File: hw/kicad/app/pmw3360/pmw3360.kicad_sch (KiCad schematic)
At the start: 13 parts, among them J1 TOP, J2 BUTTOM, U1 PMW3360DM-T2QU, U2 AMS1117-1.8

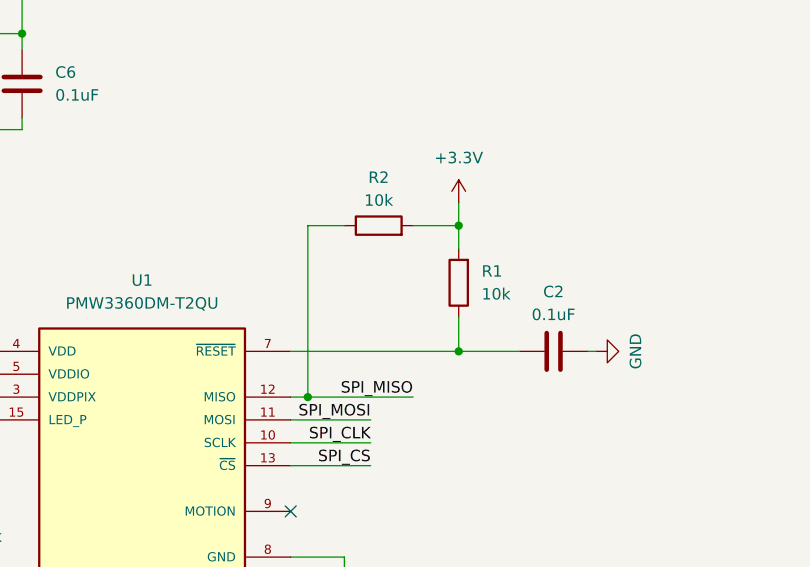
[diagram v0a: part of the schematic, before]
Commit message: Merge from normal
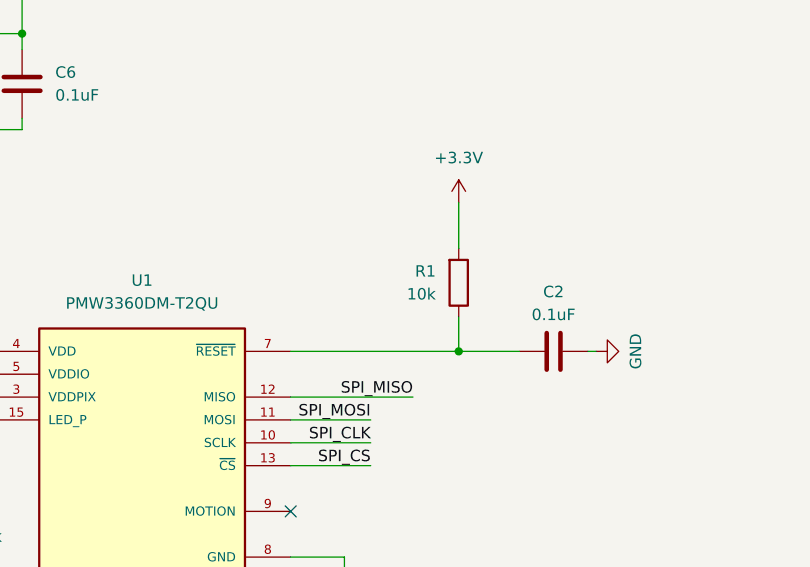
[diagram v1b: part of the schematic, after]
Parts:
- removed R2: 10k, Resistor_SMD:R_0805_2012Metric, symbol Device:R
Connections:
- net GND: now also C2.1; no longer C2.2
- net at R1.1, U1.7 (~{RESET}): now also C2.2; no longer C2.1
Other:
- moved on the sheet: C2, R1
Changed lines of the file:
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@@
 (kicad_sch (version 20230121) (generator eeschema)
   (paper "A4")
-  (junction (at 121.666 83.82) (diameter 0) (color 0 0 0 0)
-  )
   (junction (at 74.676 107.442) (diameter 0) (color 0 0 0 0)
   )
@@
   )
   (junction (at 89.916 43.434) (diameter 0) (color 0 0 0 0)
-  )
-  (junction (at 138.43 64.77) (diameter 0) (color 0 0 0 0)
   )
   (no_connect (at 119.761 96.52))
@@
     (stroke (width 0) (type default))
   )
-  (wire (pts (xy 133.35 83.82) (xy 121.666 83.82))
+  (wire (pts (xy 119.761 83.82) (xy 133.35 83.82))
     (stroke (width 0) (type default))
   )
@@
     (stroke (width 0) (type default))
   )
-  (wire (pts (xy 121.666 83.82) (xy 121.666 64.77))
-    (stroke (width 0) (type default))
-  )
   (wire (pts (xy 77.978 54.102) (xy 89.916 54.102))
     (stroke (width 0) (type default))
@@
     (stroke (width 0) (type default))
   )
-  (wire (pts (xy 133.35 64.77) (xy 138.43 64.77))
-    (stroke (width 0) (type default))
-  )
   (wire (pts (xy 231.14 80.01) (xy 240.03 80.01))
     (stroke (width 0) (type default))
@@
     (stroke (width 0) (type default))
   )
-  (wire (pts (xy 138.43 62.23) (xy 138.43 64.77))
+  (wire (pts (xy 138.43 62.23) (xy 138.43 67.31))
     (stroke (width 0) (type default))
   )
@@
     (stroke (width 0) (type default))
   )
-  (wire (pts (xy 121.666 64.77) (xy 125.73 64.77))
-    (stroke (width 0) (type default))
-  )
   (wire (pts (xy 224.79 85.09) (xy 215.9 85.09))
     (stroke (width 0) (type default))
@@
     (stroke (width 0) (type default))
   )
-  (wire (pts (xy 138.43 64.77) (xy 138.43 67.31))
-    (stroke (width 0) (type default))
-  )
   (wire (pts (xy 119.761 78.74) (xy 138.43 78.74))
     (stroke (width 0) (type default))
@@
     (stroke (width 0) (type default))
   )
-  (wire (pts (xy 121.666 83.82) (xy 119.761 83.82))
-    (stroke (width 0) (type default))
-  )
   (wire (pts (xy 63.5 41.656) (xy 63.5 43.434))
     (stroke (width 0) (type default))
@@
     )
   )
-  (symbol (lib_id "Device:R") (at 138.43 71.12 180) (unit 1)
-    (in_bom yes) (on_board yes) (dnp no) (fields_autoplaced)
-    (property "Reference" "R1" (at 140.97 69.85 0)
+  (symbol (lib_id "Device:R") (at 138.43 71.12 0) (mirror x) (unit 1)
+    (in_bom yes) (on_board yes) (dnp no)
+    (property "Reference" "R1" (at 135.89 69.85 0)
       (effects (font (size 1.27 1.27)) (justify right))
     )
-    (property "Value" "10k" (at 140.97 72.39 0)
+    (property "Value" "10k" (at 135.89 72.39 0)
       (effects (font (size 1.27 1.27)) (justify right))
     )
-    (property "Footprint" "Resistor_SMD:R_0805_2012Metric" (at 140.208 71.12 90)
+    (property "Footprint" "Resistor_SMD:R_0805_2012Metric" (at 136.652 71.12 90)
       (effects (font (size 1.27 1.27)) hide)
     )
@@
     )
   )
-  (symbol (lib_id "Device:R") (at 129.54 64.77 90) (unit 1)
-    (in_bom yes) (on_board yes) (dnp no) (fields_autoplaced)
-    (property "Reference" "R2" (at 129.54 59.436 90)
-      (effects (font (size 1.27 1.27)))
-    )
-    (property "Value" "10k" (at 129.54 61.976 90)
-      (effects (font (size 1.27 1.27)))
-    )
-    (property "Footprint" "Resistor_SMD:R_0805_2012Metric" (at 129.54 66.548 90)
-      (effects (font (size 1.27 1.27)) hide)
-    )
-    (property "Datasheet" "~" (at 129.54 64.77 0)
-      (effects (font (size 1.27 1.27)) hide)
-    )
-    (pin "1")
-    (pin "2")
-    (instances
-      (project "pmw3360"
-        (path "/988ee502-8596-4ebe-9b99-0eb76e7d156a"
-          (reference "R2") (unit 1)
-        )
-      )
-    )
-  )
   (symbol (lib_id "power:+5V") (at 63.5 41.656 0) (unit 1)
     (in_bom yes) (on_board yes) (dnp no) (fields_autoplaced)
@@
     )
   )
-  (symbol (lib_id "Device:C") (at 148.971 78.74 90) (unit 1)
-    (in_bom yes) (on_board yes) (dnp no) (fields_autoplaced)
+  (symbol (lib_id "Device:C") (at 148.971 78.74 270) (mirror x) (unit 1)
+    (in_bom yes) (on_board yes) (dnp no)
     (property "Reference" "C2" (at 148.971 72.136 90)
       (effects (font (size 1.27 1.27)))
@@
       (effects (font (size 1.27 1.27)))
     )
-    (property "Footprint" "Capacitor_SMD:C_0805_2012Metric" (at 152.781 77.7748 0)
-      (effects (font (size 1.27 1.27)) hide)
-    )
+    (property "Footprint" "Capacitor_SMD:C_0805_2012Metric" (at 145.161 77.7748 0)
+      (effects (font (size 1.27 1.27)) hide)
+    )
